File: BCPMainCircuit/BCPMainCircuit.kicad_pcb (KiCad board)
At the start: 2 copper layers, 8 parts, among them SW1 SW_Nidec_CAS-120A1, U1 LD1117V33, U2 Pico 2, U3 DEV-13712, U6 BME280

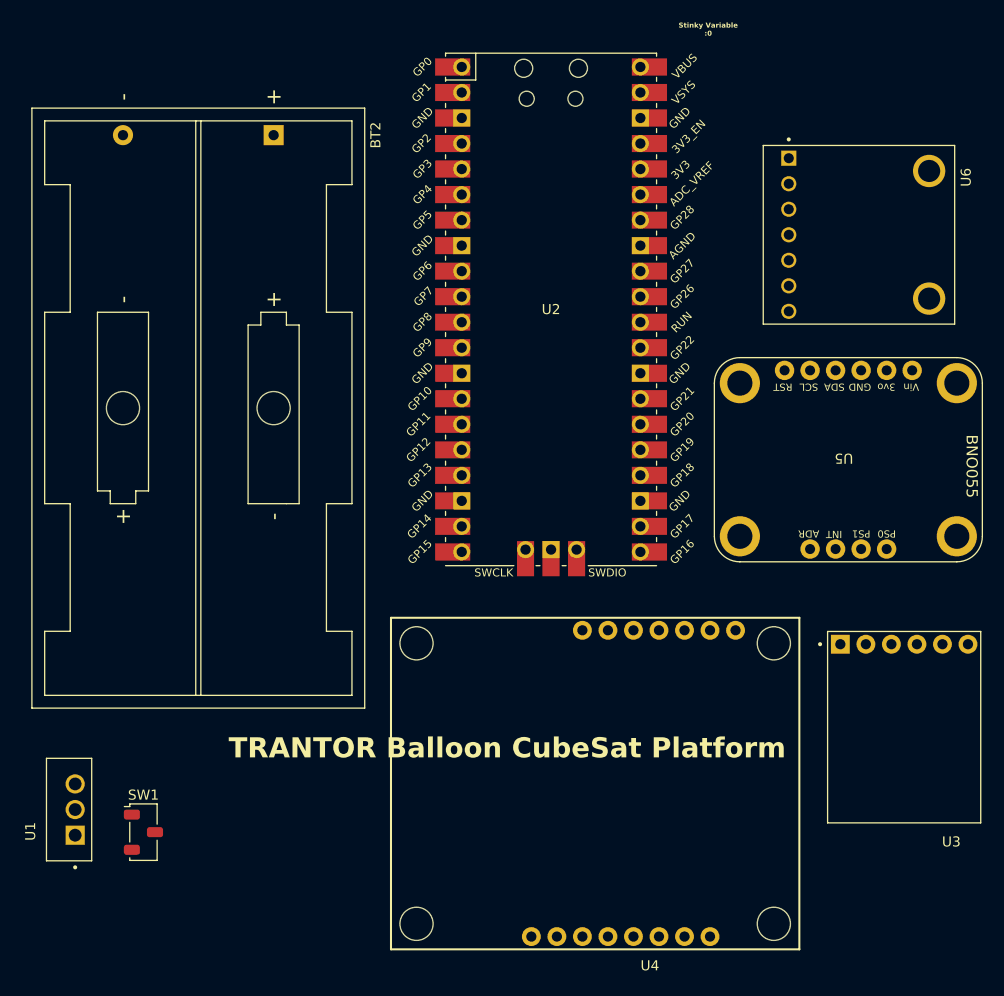
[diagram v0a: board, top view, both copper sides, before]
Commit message: Update cutout
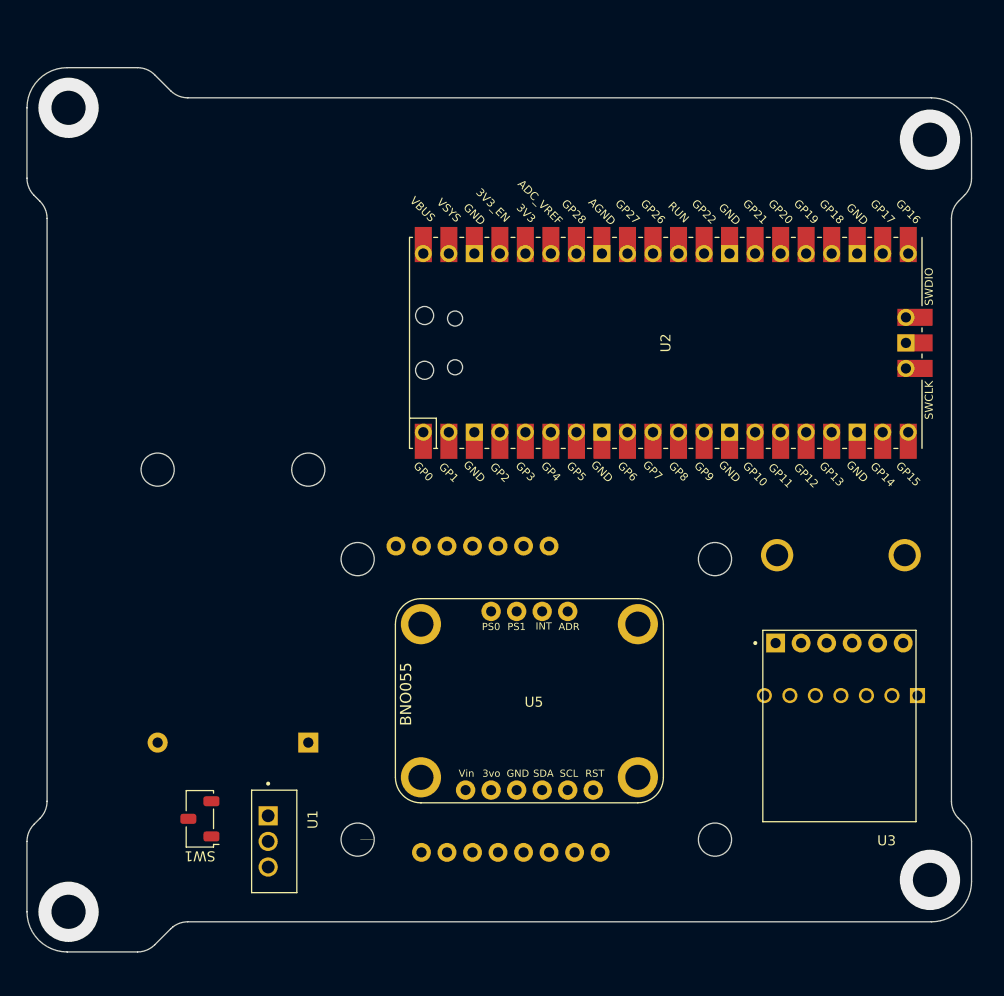
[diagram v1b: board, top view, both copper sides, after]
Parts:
- BT2, U4, U6: moved to B.Cu
- moved BT2 60.5 mm to (102.2, 99.3), turned to 90 degrees
- moved U5 39.9 mm to (124.7, 95.8), turned to 0 degrees
- moved U6 38.9 mm to (155.2, 87.6), turned to 180 degrees
- moved U4 28.0 mm to (114.4, 111.6), turned to 180 degrees
- moved U1 20.7 mm to (98.8, 109.1), turned to -90 degrees
- moved U2 11.9 mm to (137.8, 59.5), turned to 90 degrees
- moved U3 6.45 mm to (155.1, 97.6)
- moved SW1 5.77 mm to (91.4, 106.9), turned to 180 degrees
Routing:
- net (no net): vias 0 -> 4
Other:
- board outline added: 94 x 88 mm
- board text removed: "Stinky Variable :0"
